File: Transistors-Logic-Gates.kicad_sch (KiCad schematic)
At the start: 31 parts, among them J1 Conn_01x05_Socket, Q1 PN2222A, Q2 PN2222A, Q3 PN2222A, Q4 PN2222A, Q5 PN2222A, Q6 PN2222A, Q7 PN2222A, SW1 SW_SPDT, SW2 SW_SPDT, SW3 SW_SPDT, SW4 SW_SPDT, SW5 SW_Push, SW6 SW_SPDT, SW7 SW_SPDT

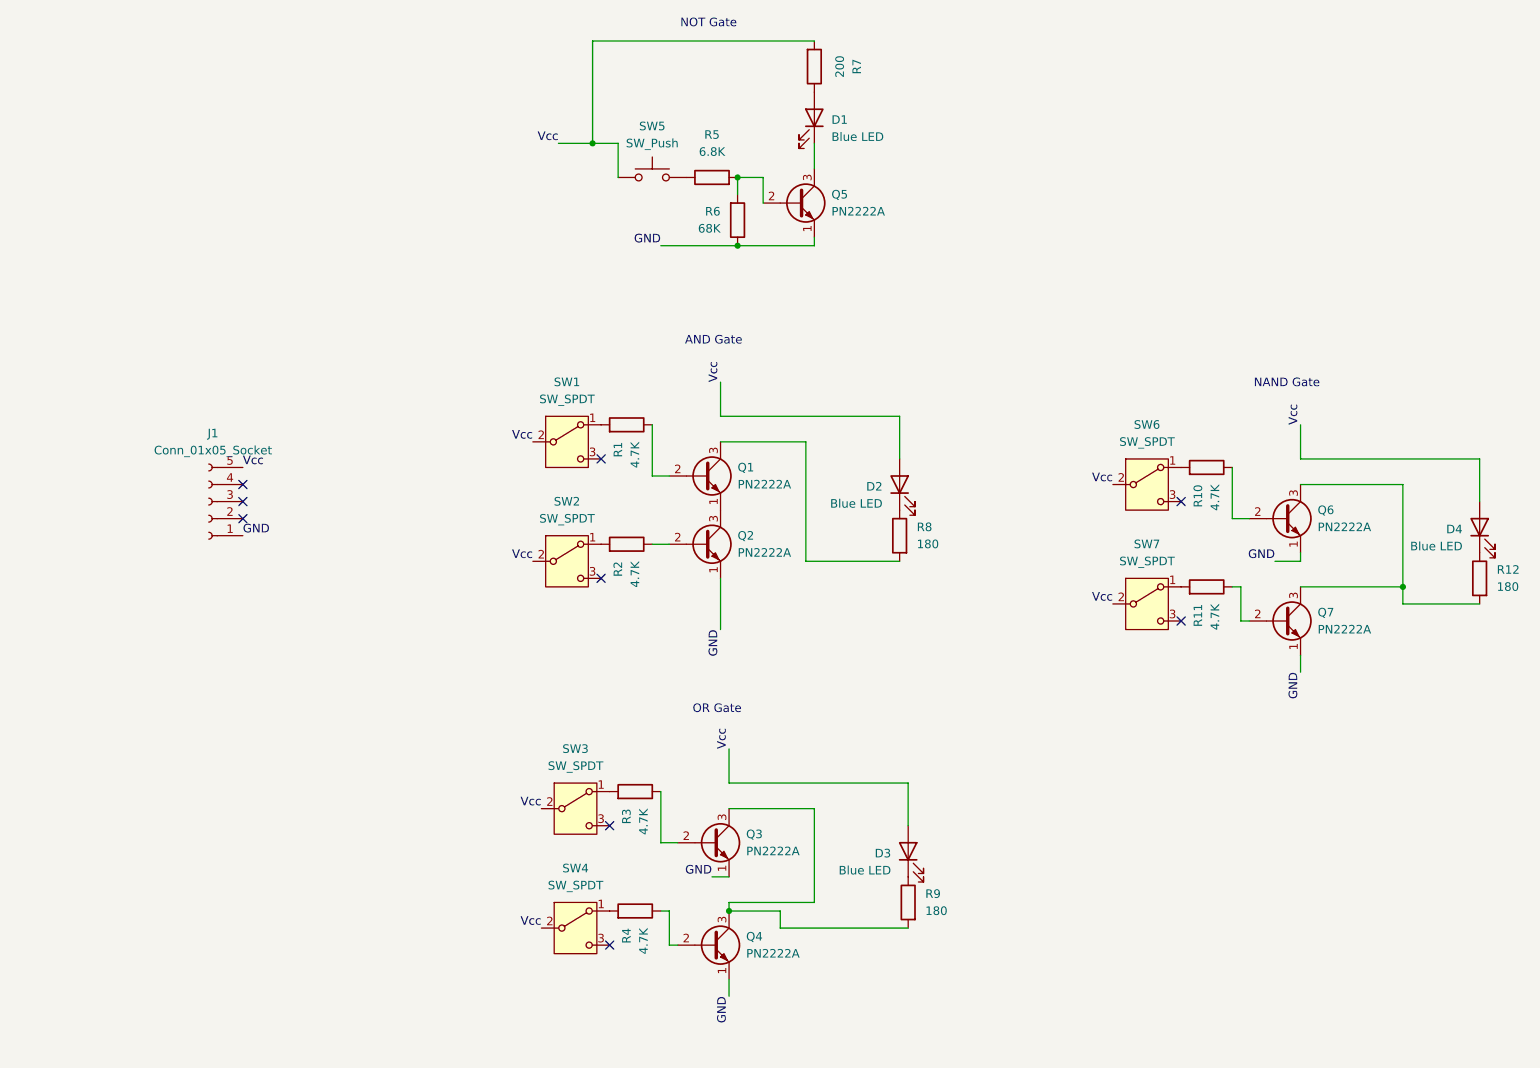
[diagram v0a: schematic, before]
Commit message: feat: first PCB made, still issue to iron out
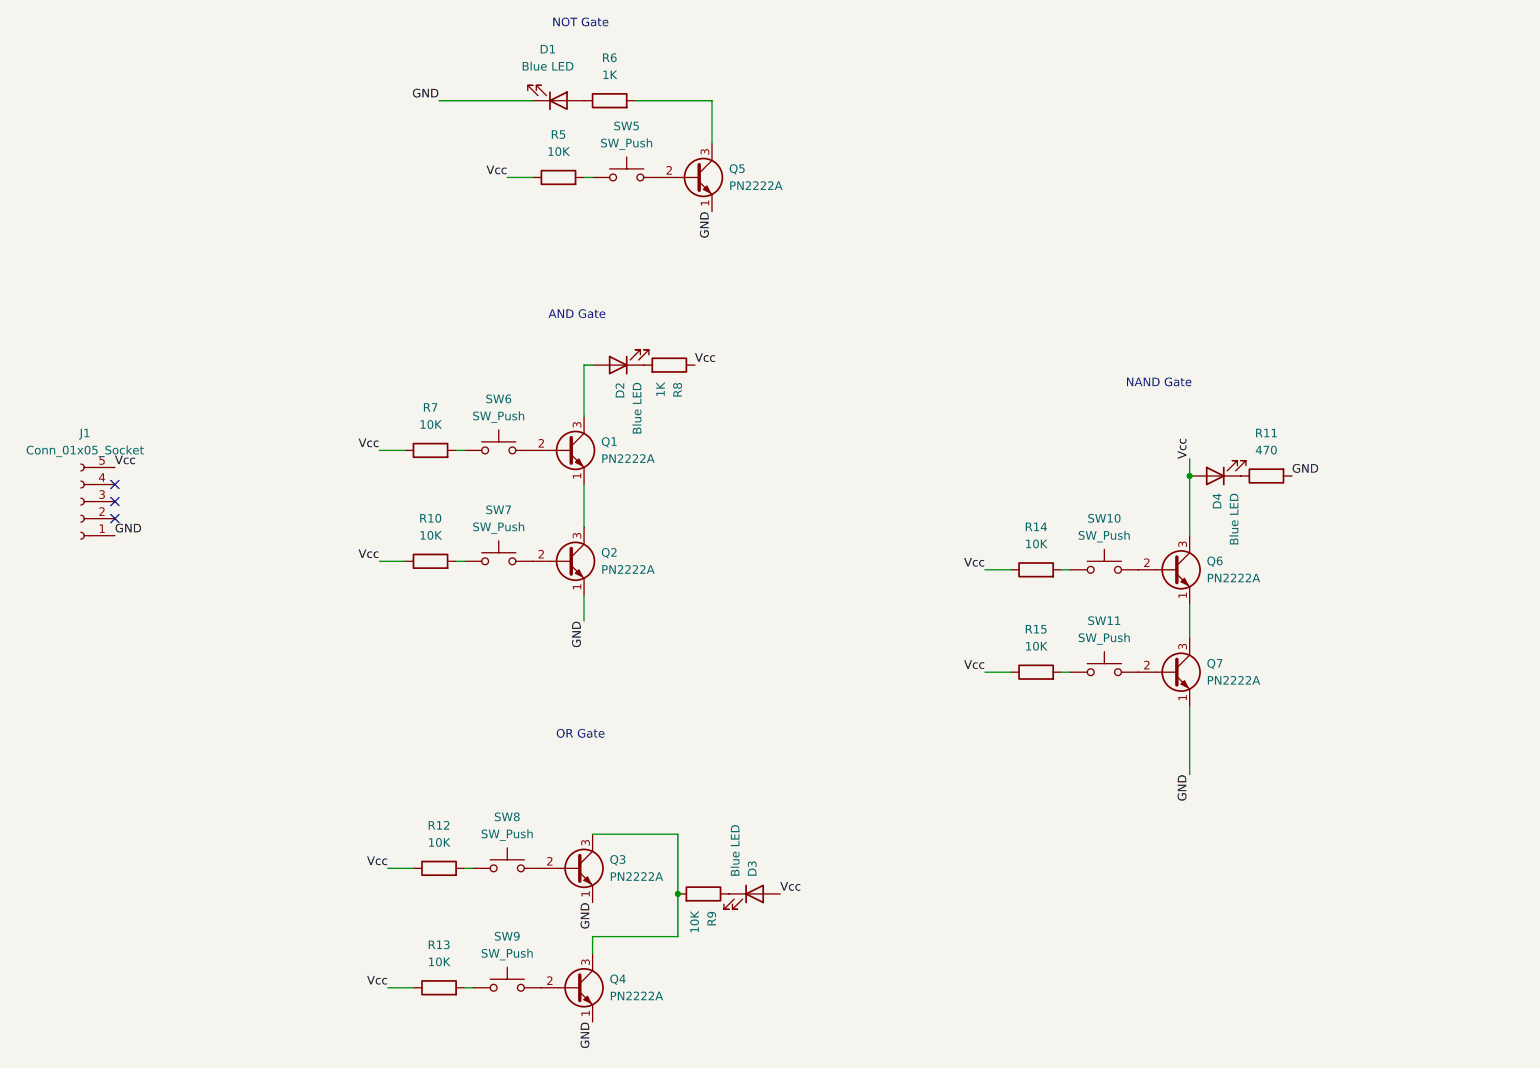
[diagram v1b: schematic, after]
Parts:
- removed R1, R2, R3, R4: 4.7K, Resistor_THT:R_Axial_DIN0204_L3.6mm_D1.6mm_P7.62mm_Horizontal, symbol Device:R
- removed SW1, SW2, SW3, SW4, SW6, SW7: SW_SPDT, Button_Switch_THT:SW_Slide-03_Wuerth-WS-SLTV_10x2.5x6.4_P2.54mm, symbol Switch:SW_SPDT
- added R13, R14, R15: 10K, Resistor_THT:R_Axial_DIN0204_L3.6mm_D1.6mm_P7.62mm_Horizontal, symbol Device:R
- added SW10, SW11, SW6, SW7, SW8, SW9: SW_Push, Button_Switch_THT:SW_PUSH_6mm_H5mm, symbol Switch:SW_Push
- R10: value 4.7K -> 10K
- R11: value 4.7K -> 470
- R12, R9: value 180 -> 10K
- R5: value 6.8K -> 10K
- R6: value 68K -> 1K
- R7: value 200 -> 10K
- R8: value 180 -> 1K
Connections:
- net GND: now also D1.1 (K), R11.2; no longer Q6.1 (E), R6.1
- net Vcc: now also Q6.3 (C), R10.1, R12.1, R5.1, R7.1, R8.1, R13.1, R14.1, R15.1; no longer D2.2 (A), R7.2, SW5.1
- net at Q3.2 (B): now also SW8.2
- net at Q6.2 (B): now also SW10.2; no longer R10.1
- net at Q2.2 (B): now also SW7.2
- net at Q1.2 (B): now also SW6.2
- net at Q1.3 (C): now also D2.2 (A); no longer R8.2
- net at D1.2 (A): now also R6.1; no longer R7.1
- net at Q7.2 (B): now also SW11.2; no longer R11.1
- net at Q4.2 (B): now also SW9.2
- net at SW5.2: now also Q5.2 (B); no longer R5.1
- net at D2.1 (K): now also R8.2; no longer R8.1
- net at R10.2: now also SW7.1
- net at Q5.3 (C): now also R6.2; no longer D1.1 (K)
- net at D4.1 (K): now also R11.1; no longer R12.1
- new net: Q6.1 (E), Q7.3 (C)
- new net: R12.2, SW8.1
- new net: R5.2, SW5.1
- new net: R14.2, SW10.1
- new net: R15.2, SW11.1
- new net: R13.2, SW9.1
- new net: R7.2, SW6.1
- no-connect marks 9 -> 3
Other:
- moved on the sheet: D1, D2, D3, J1, Q1, Q2, Q3, Q4, Q5, R8, R9, SW5
